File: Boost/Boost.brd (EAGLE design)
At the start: 100 x 80 mm, 2 parts

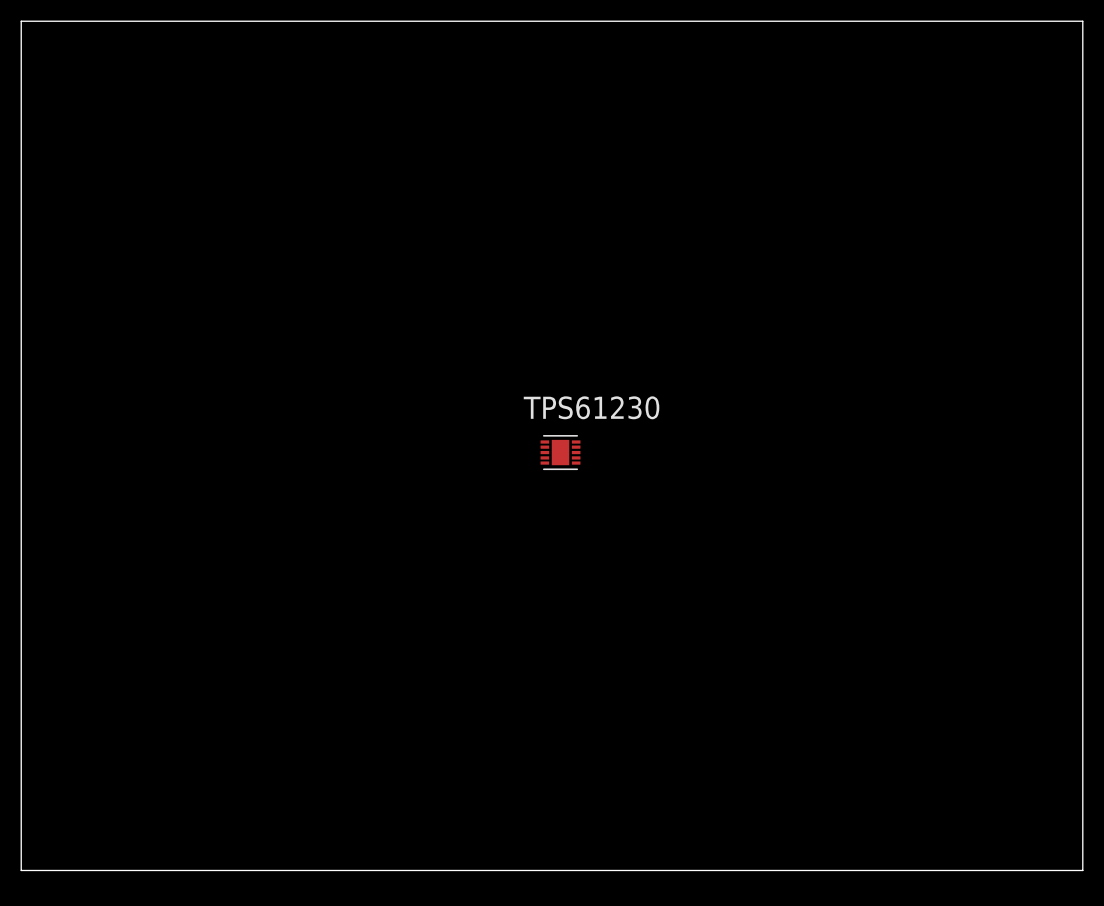
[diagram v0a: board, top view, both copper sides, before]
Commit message: boost
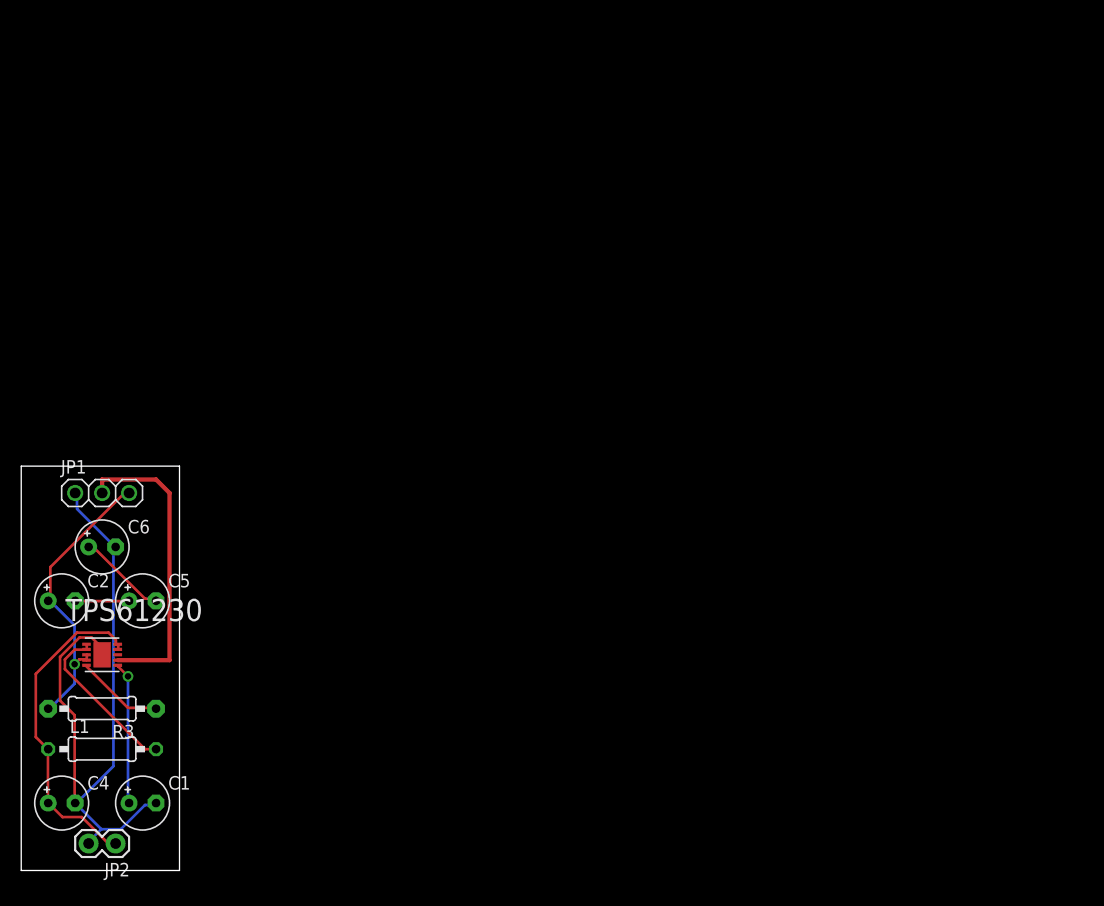
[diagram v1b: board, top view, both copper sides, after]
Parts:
- added C1: 10nF, adafruit:E2,5-5
- added C2, C4, C5, C6: 22uF, adafruit:E2,5-5
- added JP1: (no value), adafruit:1X03
- added JP2: M02PTH, SparkFun-Connectors:1X02
- added L1: 1uH, eagle-ltspice:0207/10
- added R3: 1M Ohm, adafruit:0207/10
- moved TPS61230 47.2 mm to (7.62, 20.3)
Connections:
- new net N$1: C1.-, C4.-, C6.-, JP1.1, JP2.2, TPS61230.11
- new net N$10: C2.-, C5.+
- new net N$2: R3.1, TPS61230.5
- new net N$3: L1.2, TPS61230.1, TPS61230.2
- new net N$4: C2.+, JP1.3, R3.2, TPS61230.3, TPS61230.4
- new net N$5: JP1.2, TPS61230.7
- new net N$7: C1.+, TPS61230.6
- new net N$8: C4.+, JP2.1, L1.1, TPS61230.10, TPS61230.9
- new net N$9: C5.-, C6.+
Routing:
- net N$1: track 0.00 -> 64.2 mm
- net N$8: track 0.00 -> 31.3 mm
- net N$5: track 0.00 -> 28.8 mm
- net N$4: track 0.00 -> 27.8 mm, vias 0 -> 1
- net N$3: track 0.00 -> 15.6 mm
- net N$7: track 0.00 -> 13.4 mm, vias 0 -> 1
- net N$9: track 0.00 -> 8.49 mm
- net N$2: track 0.00 -> 8.29 mm
- net N$10: track 0.00 -> 5.08 mm
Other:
- board size 100 x 80 mm -> 14.9 x 38.1 mm
